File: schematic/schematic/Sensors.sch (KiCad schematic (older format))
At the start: 13 parts, among them J1 Conn_01x05, J11 Conn_01x07, J12 Conn_01x07, J4 Conn_01x05, U9 INA219AIDCNR

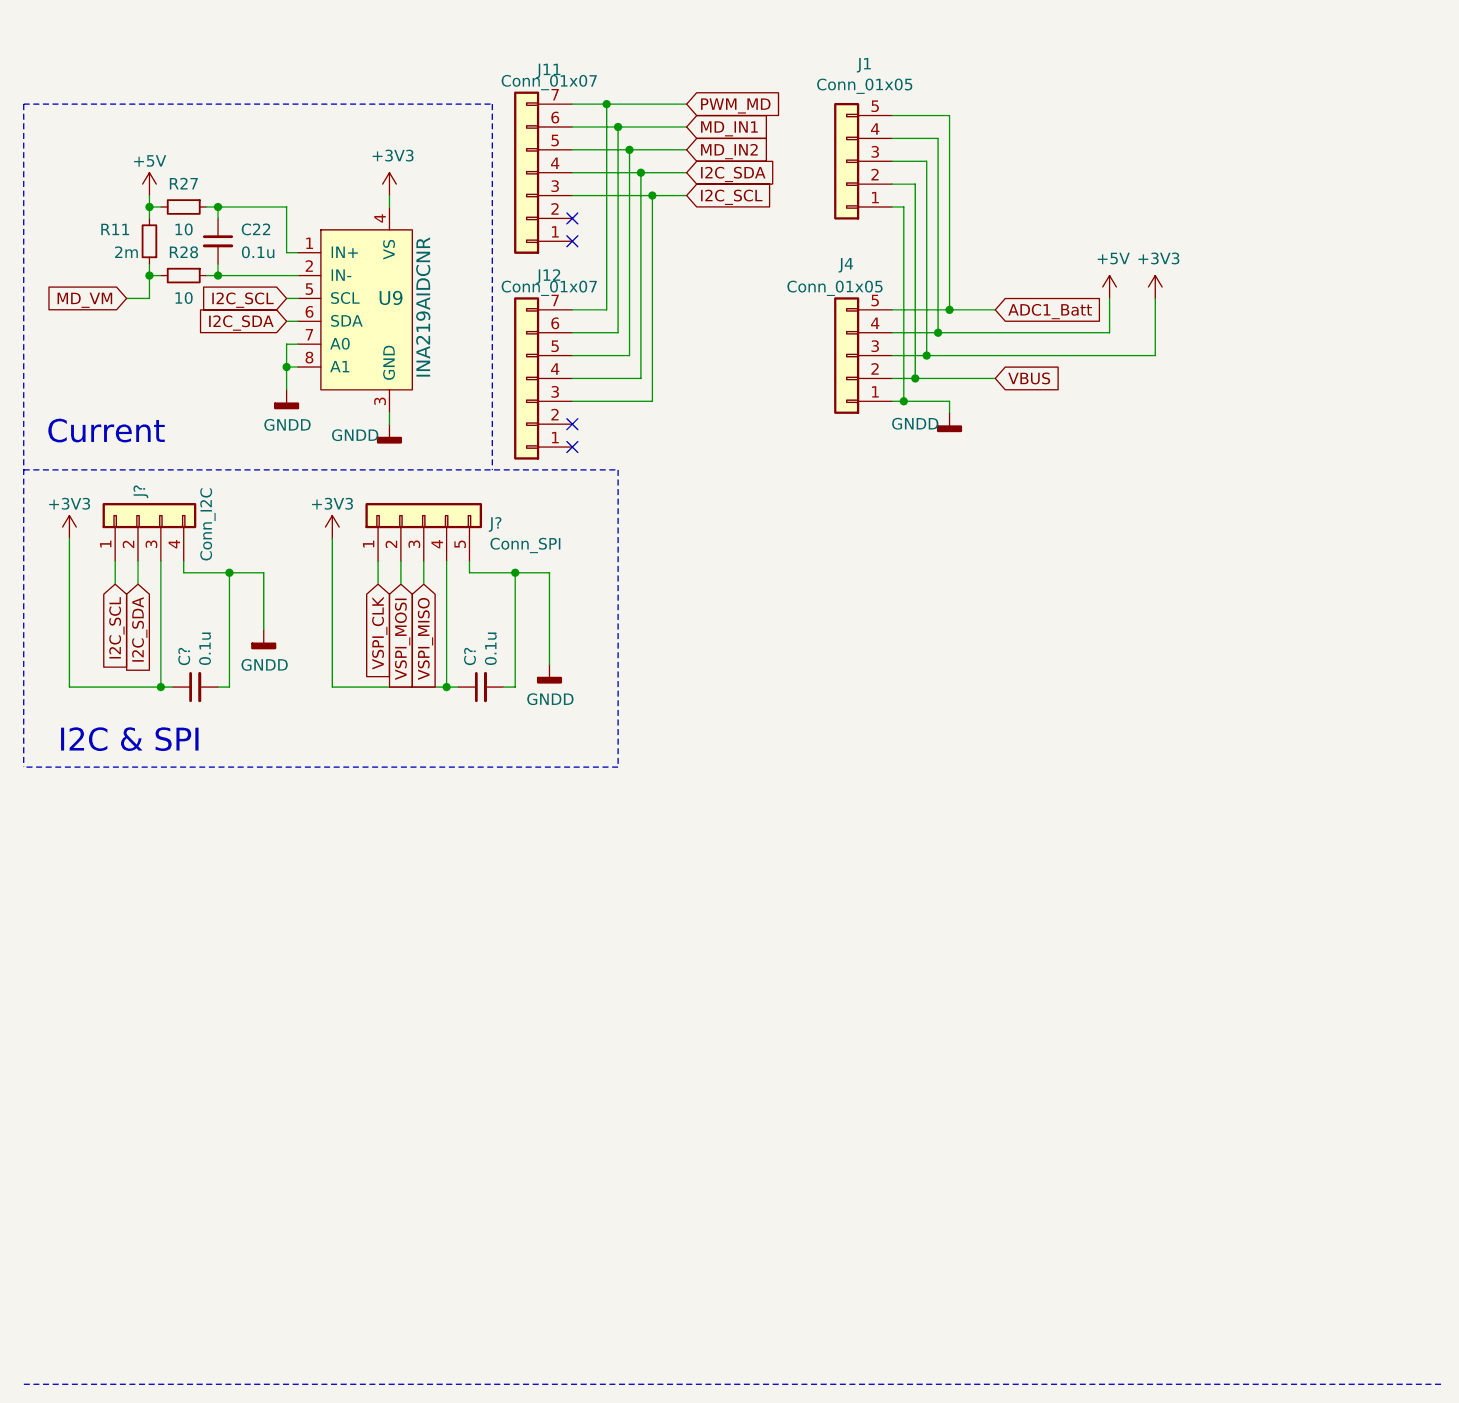
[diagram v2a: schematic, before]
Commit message: ちょっとシンプルにしよう
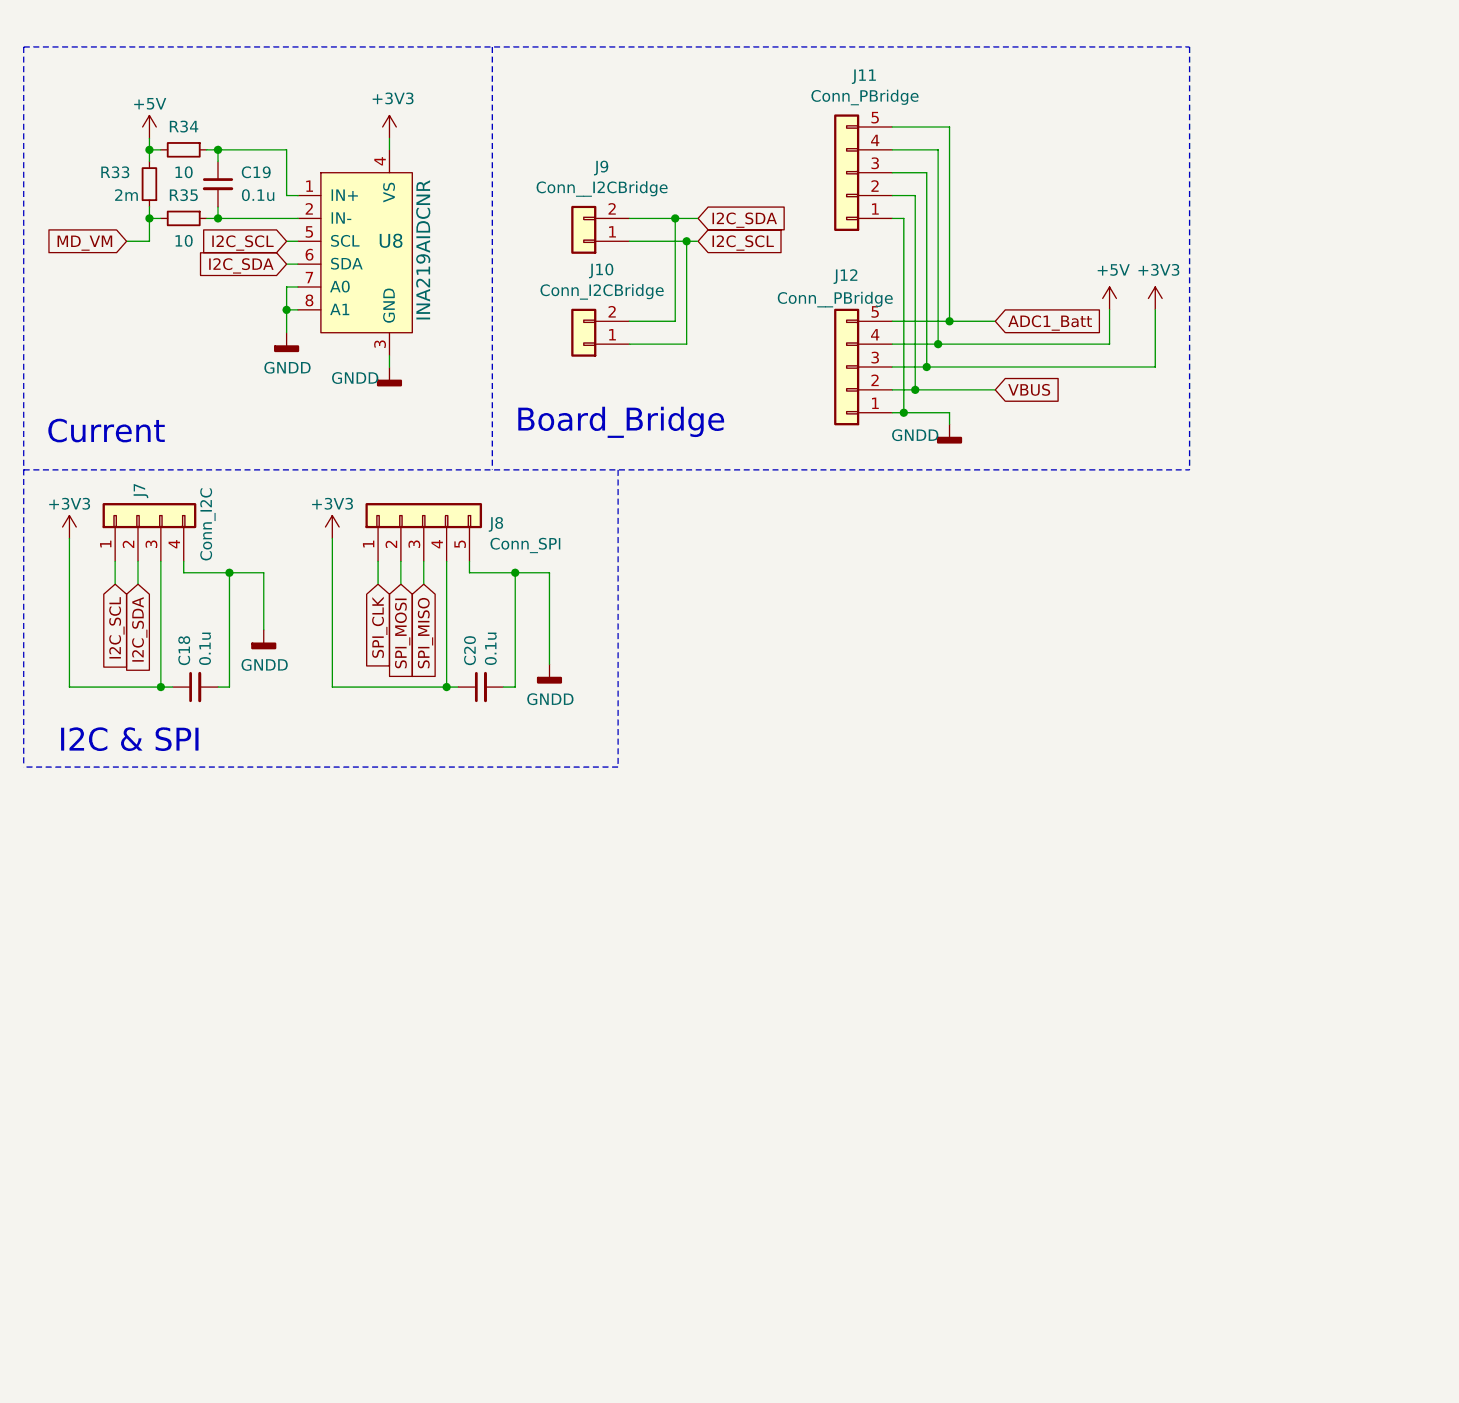
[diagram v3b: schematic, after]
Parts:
- removed J11, J12: Conn_01x07, Connector_PinHeader_1.00mm:PinHeader_2x04_P1.00mm_Vertical_SMD, symbol Connector_Generic:Conn_01x07
- added J10: Conn_I2CBridge, symbol Connector_Generic:Conn_01x02
- added J9: Conn__I2CBridge, symbol Connector_Generic:Conn_01x02
- J11: renamed from J1; value Conn_01x05 -> Conn_PBridge
- J12: renamed from J4; value Conn_01x05 -> Conn__PBridge
- gave numbers to parts that had none: 4
- renumbered C22 to C19, R11 to R33, R27 to R34, R28 to R35, U9 to U8
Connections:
- net I2C_SCL: now also J10.1 (Pin_1), J9.1 (Pin_1)
- net I2C_SDA: now also J10.2 (Pin_2), J9.2 (Pin_2)
- net VSPI_CLK renamed SPI_CLK
- net VSPI_MISO renamed SPI_MISO
- net VSPI_MOSI renamed SPI_MOSI
- no-connect marks 4 -> 0
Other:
- note added: "Board_Bridge"
- moved on the sheet: C19, J11, J12, R33, R34, R35, U8

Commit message: Change MD to DRV8830
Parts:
- J10, J9: footprint (none) -> Connector_PinHeader_1.00mm:PinHeader_2x03_P1.00mm_Vertical_SMD
- J8: footprint (none) -> Connector_PinSocket_2.54mm:PinSocket_1x05_P2.54mm_Vertical
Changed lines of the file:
@@
 F 0 "J9" H 2970 1125 50  0000 C CNN
 F 1 "Conn__I2CBridge" H 2970 1216 50  0000 C CNN
-F 2 "" H 3050 1450 50  0001 C CNN
+F 2 "Connector_PinHeader_1.00mm:PinHeader_2x03_P1.00mm_Vertical_SMD" H 3050 1450 50  0001 C CNN
 F 3 "~" H 3050 1450 50  0001 C CNN
 	1    3050 1450
@@
 F 0 "J10" H 2970 1575 50  0000 C CNN
 F 1 "Conn_I2CBridge" H 2970 1666 50  0000 C CNN
-F 2 "" H 3050 1900 50  0001 C CNN
+F 2 "Connector_PinHeader_1.00mm:PinHeader_2x03_P1.00mm_Vertical_SMD" H 3050 1900 50  0001 C CNN
 F 3 "~" H 3050 1900 50  0001 C CNN
 	1    3050 1900
@@
 F 0 "J8" V 2316 2362 50  0000 R CNN
 F 1 "Conn_SPI" V 2225 2362 50  0000 R CNN
-F 2 "" H 2350 2650 50  0001 C CNN
+F 2 "Connector_PinSocket_2.54mm:PinSocket_1x05_P2.54mm_Vertical" H 2350 2650 50  0001 C CNN
 F 3 "~" H 2350 2650 50  0001 C CNN
 	1    2350 2650
